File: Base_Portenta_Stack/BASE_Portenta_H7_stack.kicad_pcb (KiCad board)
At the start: 2 copper layers, 84.2 x 26.7 mm, 23 parts, among them J4 PinHeader_1x04_P2.00mm_Vertic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, U1 ABX00042

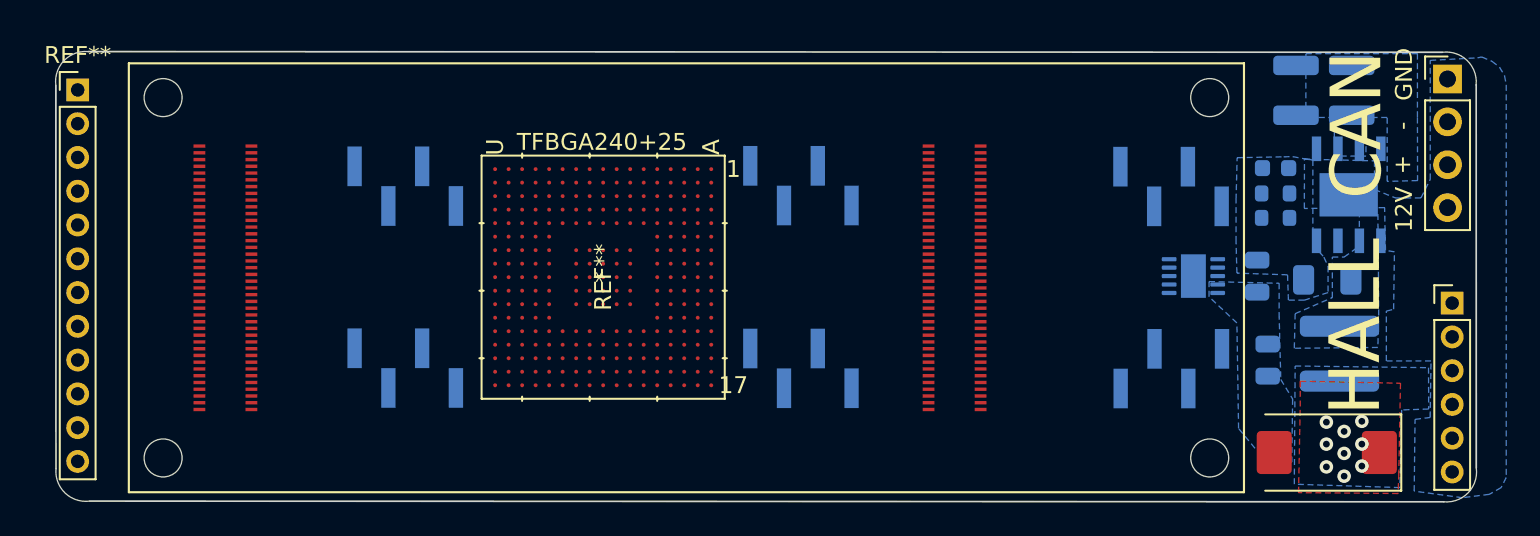
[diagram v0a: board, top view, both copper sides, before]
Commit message: Aligned
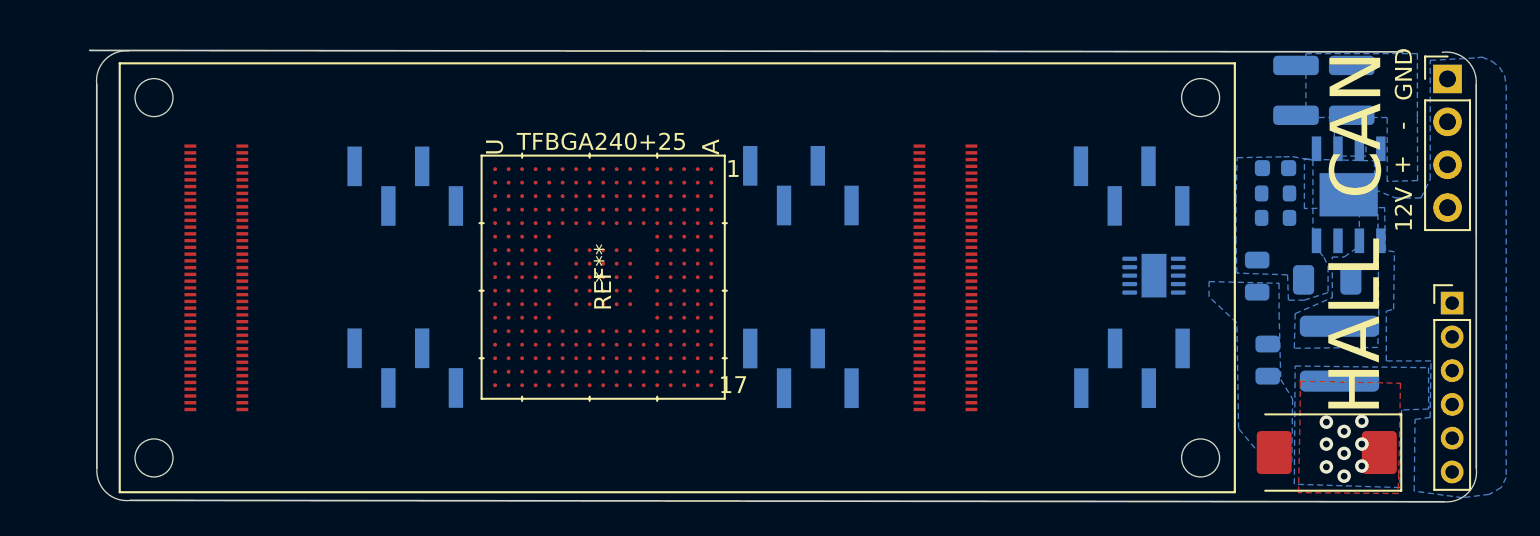
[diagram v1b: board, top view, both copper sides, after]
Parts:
- removed the REF** at (101.6, 82.7)
- moved J4 2.34 mm to (164.0, 88.4)
- moved J4 2.34 mm to (164.0, 99.2)
- moved REF** 2.34 mm to (165.3, 93.7)
- moved U1 0.54 mm to (137.1, 93.8)
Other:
- board size 84.2 x 26.7 mm -> 82.1 x 26.7 mm
